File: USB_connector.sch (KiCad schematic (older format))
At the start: 1 part, among them J1 USB_B_Micro

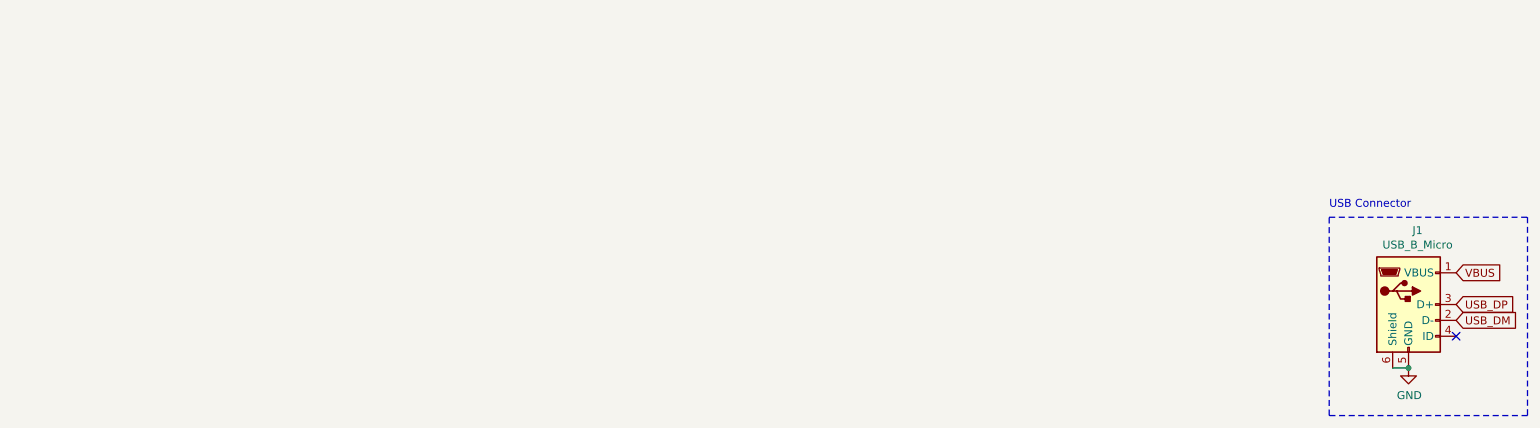
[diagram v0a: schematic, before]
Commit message: Ready to order
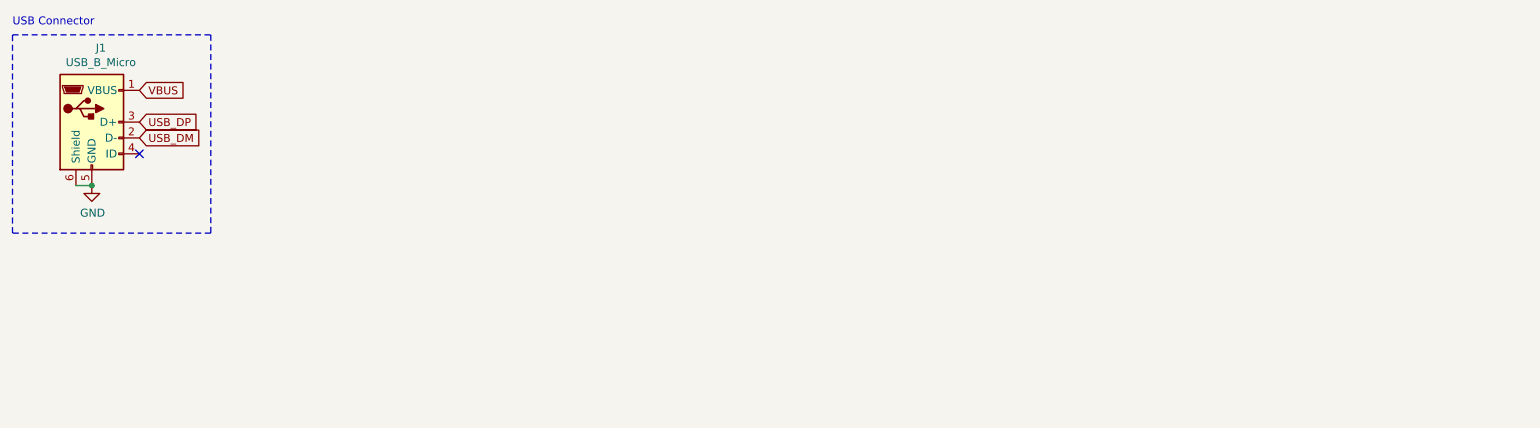
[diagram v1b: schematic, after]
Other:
- moved on the sheet: J1
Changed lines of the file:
@@
 L Connector:USB_B_Micro J1
 U 1 1 5FFB1BCE
-P 9600 4900
-F 0 "J1" H 9657 5367 50  0000 C CNN
-F 1 "USB_B_Micro" H 9657 5276 50  0000 C CNN
-F 2 "Connector_USB:USB_Micro-B_Amphenol_10104110_Horizontal" H 9750 4850 50  0001 C CNN
-F 3 "~" H 9750 4850 50  0001 C CNN
-	1    9600 4900
+P 1300 3750
+F 0 "J1" H 1357 4217 50  0000 C CNN
+F 1 "USB_B_Micro" H 1357 4126 50  0000 C CNN
+F 2 "Connector_USB:USB_Micro-B_Amphenol_10104110_Horizontal" H 1450 3700 50  0001 C CNN
+F 3 "~" H 1450 3700 50  0001 C CNN
+	1    1300 3750
 	1    0    0    -1
 $EndComp
@@
 L power:GND #PWR0101
 U 1 1 5FFB1BD4
-P 9600 5300
-F 0 "#PWR0101" H 9600 5050 50  0001 C CNN
-F 1 "GND" H 9605 5127 50  0000 C CNN
-F 2 "" H 9600 5300 50  0001 C CNN
-F 3 "" H 9600 5300 50  0001 C CNN
-	1    9600 5300
+P 1300 4150
+F 0 "#PWR0101" H 1300 3900 50  0001 C CNN
+F 1 "GND" H 1305 3977 50  0000 C CNN
+F 2 "" H 1300 4150 50  0001 C CNN
+F 3 "" H 1300 4150 50  0001 C CNN
+	1    1300 4150
 	1    0    0    -1
 $EndComp
-Text GLabel 9900 5000 2    50   Input ~ 0
+Text GLabel 1600 3850 2    50   Input ~ 0
 USB_DM
-Text GLabel 9900 4900 2    50   Input ~ 0
+Text GLabel 1600 3750 2    50   Input ~ 0
 USB_DP
 Wire Wire Line
-	9500 5300 9600 5300
-Connection ~ 9600 5300
-NoConn ~ 9900 5100
-Text GLabel 9900 4700 2    50   Input ~ 0
+	1200 4150 1300 4150
+Connection ~ 1300 4150
+NoConn ~ 1600 3950
+Text GLabel 1600 3550 2    50   Input ~ 0
 VBUS
-Text Notes 9100 4300 0    50   ~ 0
+Text Notes 800  3150 0    50   ~ 0
 USB Connector
 Wire Notes Line
-	9100 4350 10350 4350
+	800  3200 2050 3200
 Wire Notes Line
-	10350 4350 10350 5600
+	2050 3200 2050 4450
 Wire Notes Line
-	10350 5600 9100 5600
+	2050 4450 800  4450
 Wire Notes Line
-	9100 5600 9100 4350
+	800  4450 800  3200
 $EndSCHEMATC
